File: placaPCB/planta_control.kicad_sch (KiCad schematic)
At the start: 55 parts, among them J1 Conn_01x15_Pin, J2 USB_C_Receptacle, J3 Conn_01x15_Pin, J4 Conn_01x04_Pin, J5 Conn_01x06_Pin, J6 Conn_01x02_Pin, J7 Conn_01x02_Pin, Q1 MMBT3904, Q2 MMBT3904, SW1 SW_DIP_x01, T1 TIP31C, T2 TIP31C, U1 ESp32, U2 LM358, U3 DS18B20, U4 DS18B20, U5 DS18B20Z, U6 DS18B20Z

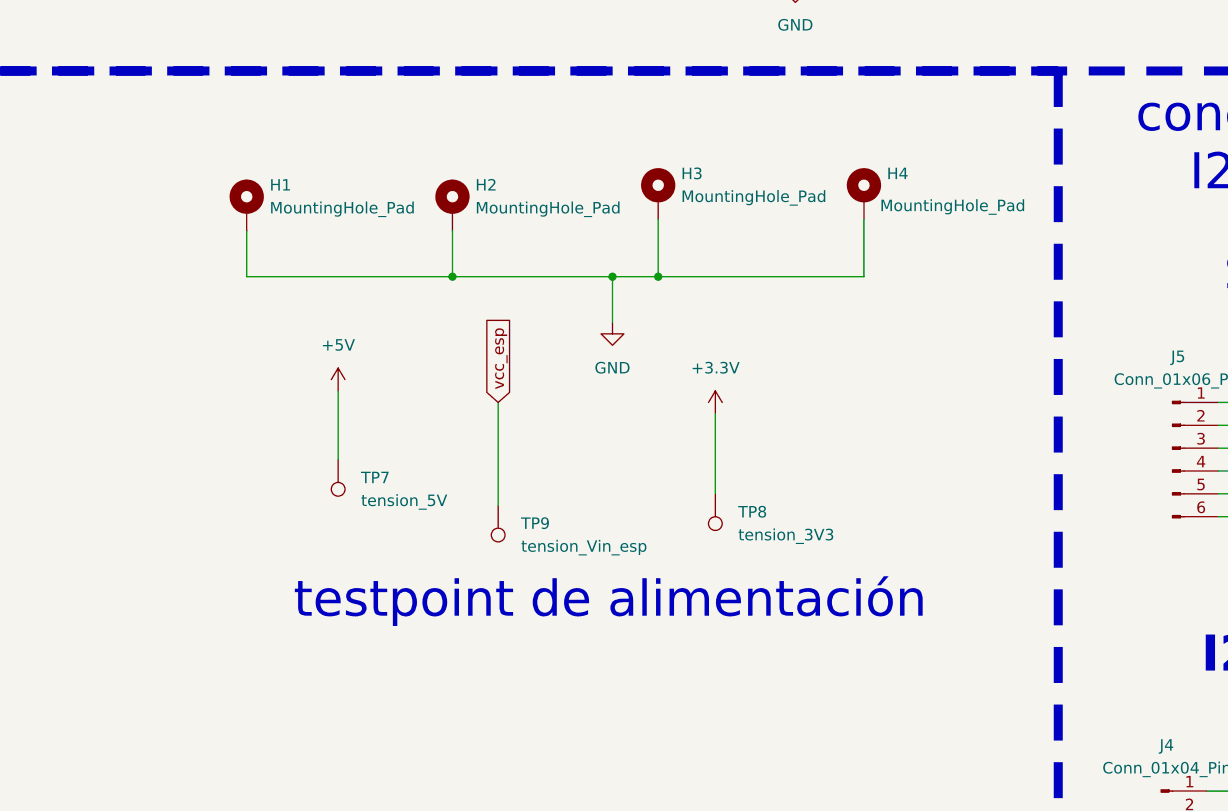
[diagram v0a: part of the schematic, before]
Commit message: .
.
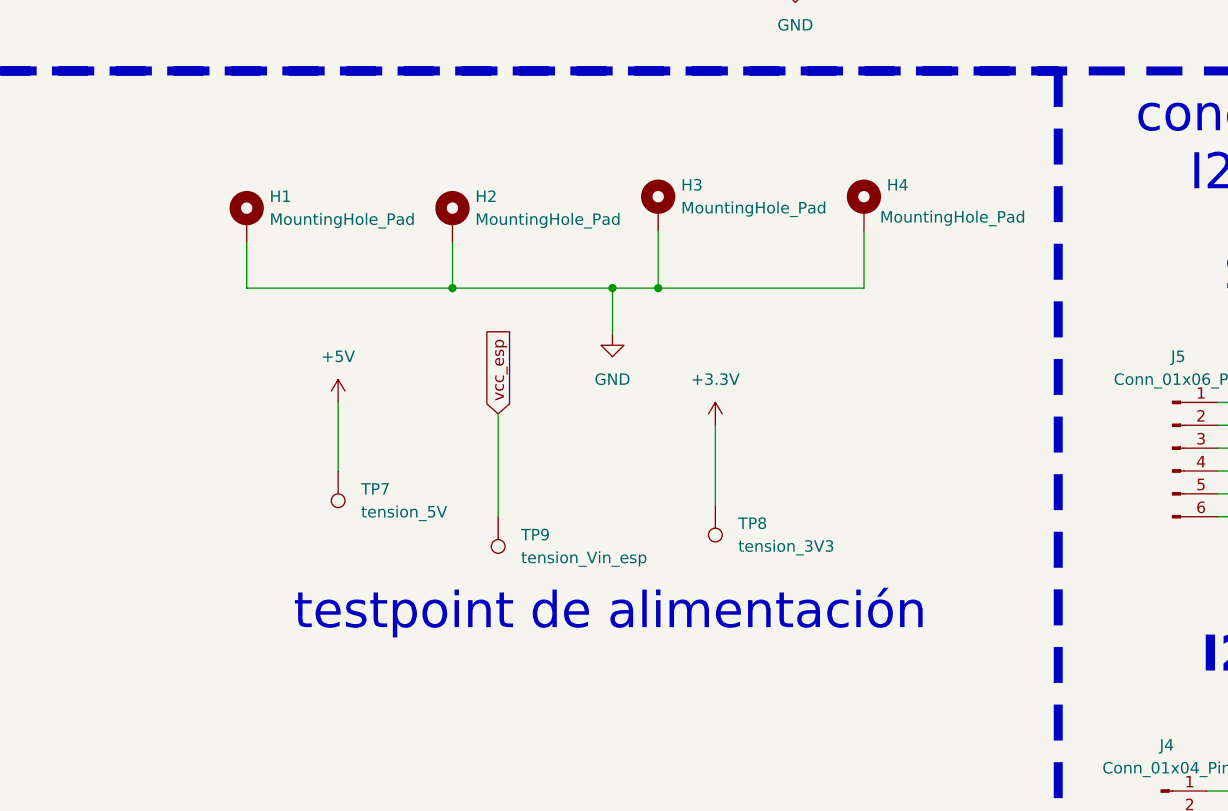
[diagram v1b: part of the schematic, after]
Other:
- moved on the sheet: H1, H2, H3, H4, TP7, TP8, TP9
